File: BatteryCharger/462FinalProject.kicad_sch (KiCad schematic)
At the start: 45 parts, among them IC1 TPS562231DRLR, J1 Conn_01x05_Pin, J2 Conn_01x03_Pin, J3 USB_B_Micro, Q1 MMFTN6001, Q2 MMFTN6001, Q3 MMFTN6001, Q4 MMFTN6001, Q5 MMFTN6001, Q6 BSS84AK,215, Q7 BSS84AK,215, Q8 BSS84AK,215, U1 MIC5504-3.3YM5, U2 STM32G030F6Px

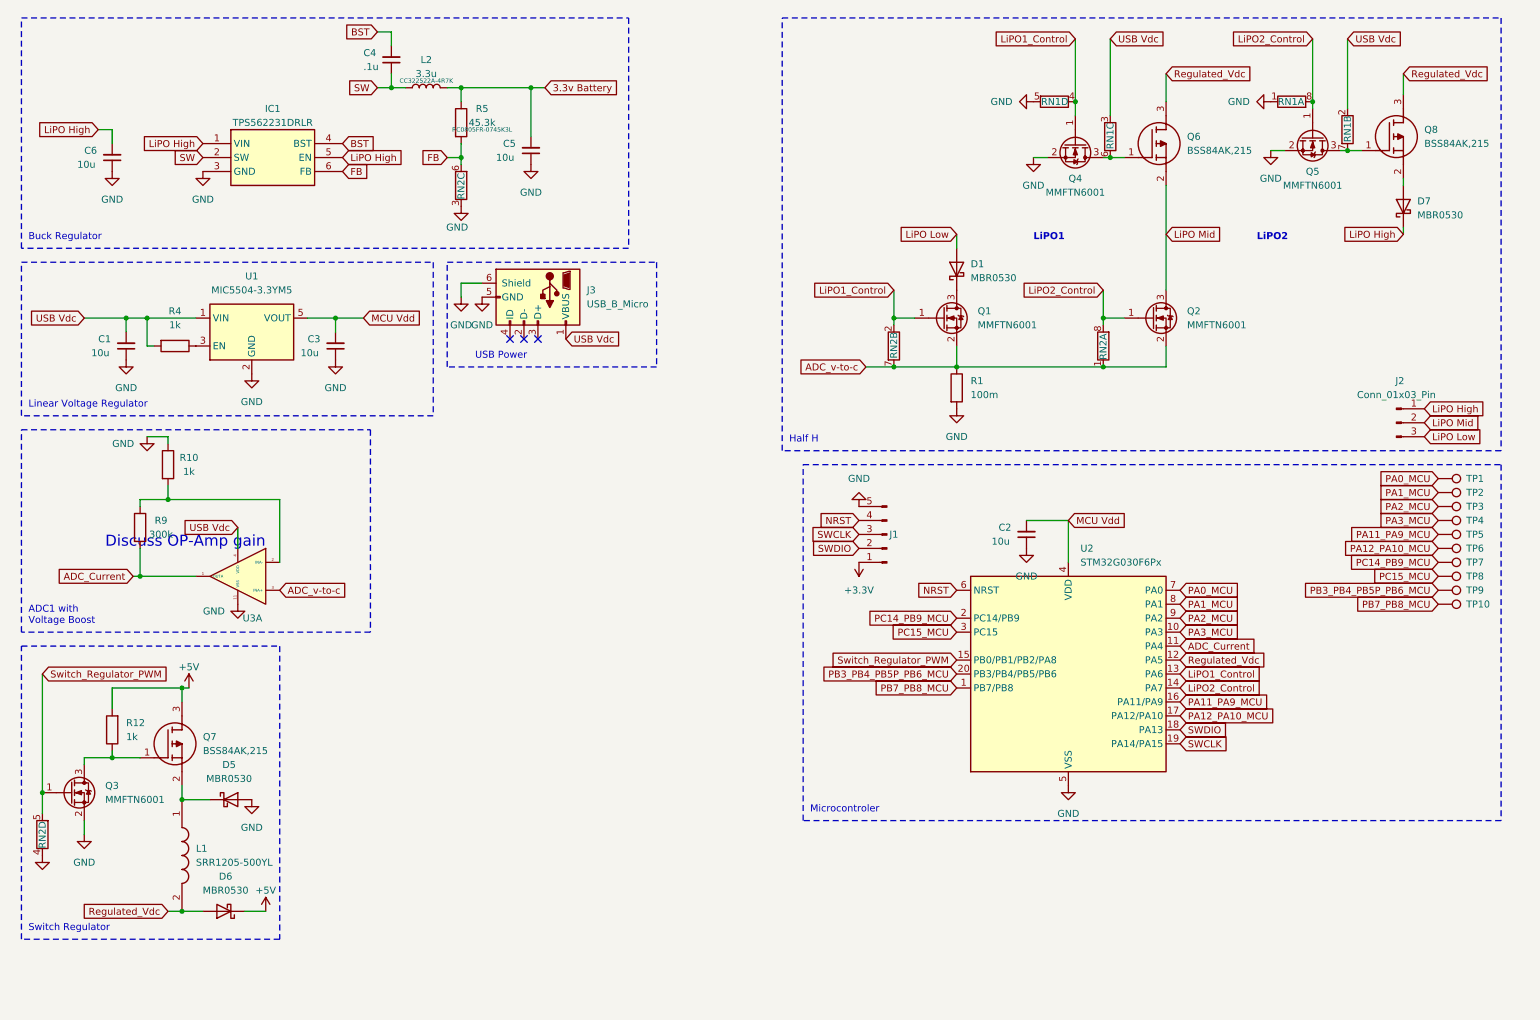
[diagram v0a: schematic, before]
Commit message: commit
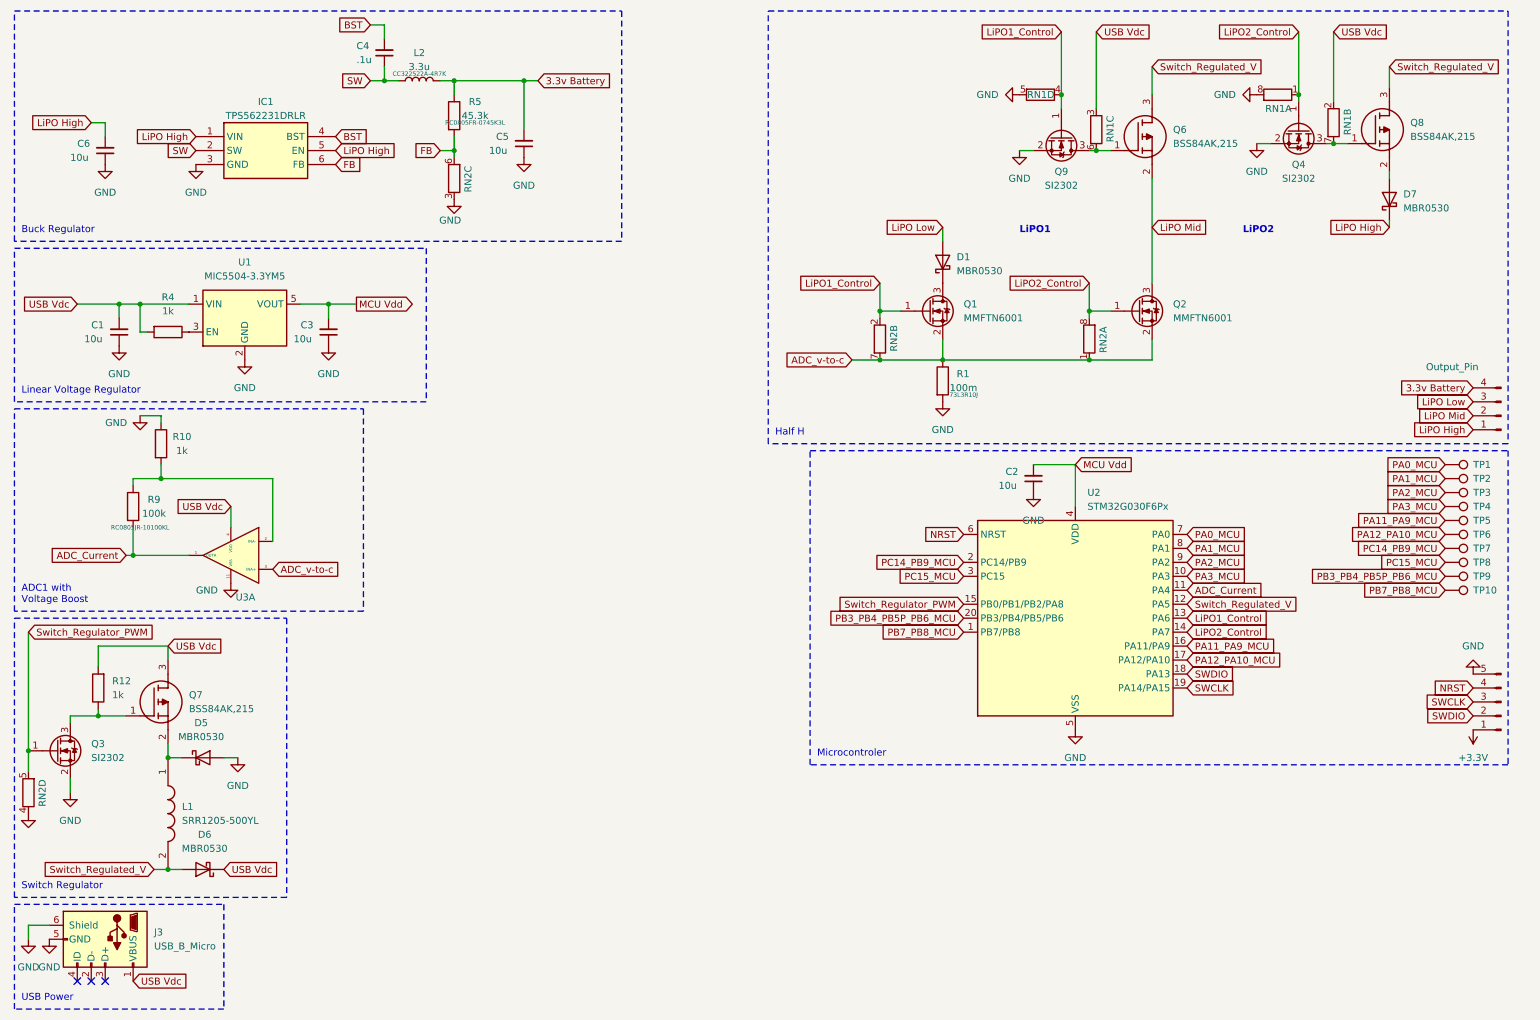
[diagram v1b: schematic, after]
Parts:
- removed Q5: MMFTN6001, Package_TO_SOT_SMD:SOT-23, symbol Device:Q_NMOS_GSD
- added Q9: SI2302, Package_TO_SOT_SMD:SOT-23, symbol Device:Q_NMOS_GSD
- J2: value Conn_01x03_Pin -> Output_Pin; symbol Connector:Conn_01x03_Pin -> Connector:Conn_01x04_Pin
- Q3, Q4: value MMFTN6001 -> SI2302; Manufacturer Diotec Semiconductor -> (none); Manufacturer Part Number MMFTN6001 -> (none); Mouser Part Number 637-MMFTN6001 -> (none); Mouser Price/Stock https://www.mouser.com/ProductDetail/Diotec-Semiconductor/M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 -> (none)
- R9: value 300k -> 100k
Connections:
- net +5V is gone; now on net USB Vdc: D6.1 (K), Q7.3 (D), R12.2
- net 3.3v Battery: now also J2.4 (Pin_4)
- net GND: now also RN1.8 (R1.2), Q9.2 (S); no longer RN1.1 (R1.1)
- net LiPO1_Control: now also Q9.1 (G); no longer Q4.1 (G)
- net LiPO2_Control: now also Q4.1 (G), RN1.1 (R1.1); no longer RN1.8 (R1.2)
- net at Q6.1 (G), RN1.6 (R3.2): now also Q9.3 (D); no longer Q4.3 (D)
- net at Q8.1 (G), RN1.7 (R2.2): now also Q4.3 (D)
- net Regulated_Vdc renamed Switch_Regulated_V
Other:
- note removed: "Discuss OP-Amp gain"
- moved on the sheet: C1, C2, C3, C4, C5, C6, D1, D5, D6, D7, IC1, J3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
